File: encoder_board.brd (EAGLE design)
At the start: 39 x 43.2 mm, 13 parts, among them J1 1X2-3.5MM, J2 1X2-3.5MM, J3 1X2-3.5MM, Q1 BSS138, Q2 BSS138, Q3 BSS138, U1 ATTINY85-20P

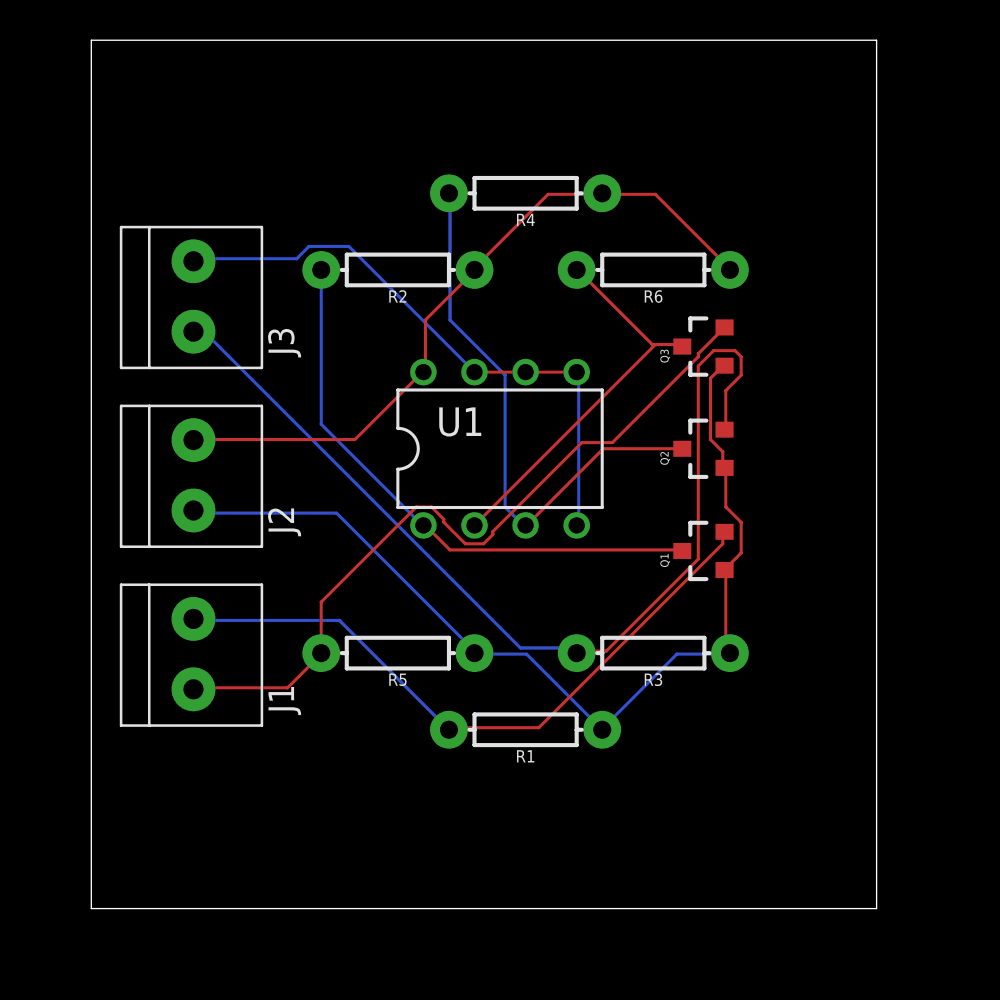
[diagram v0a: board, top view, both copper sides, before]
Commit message: Add files via upload
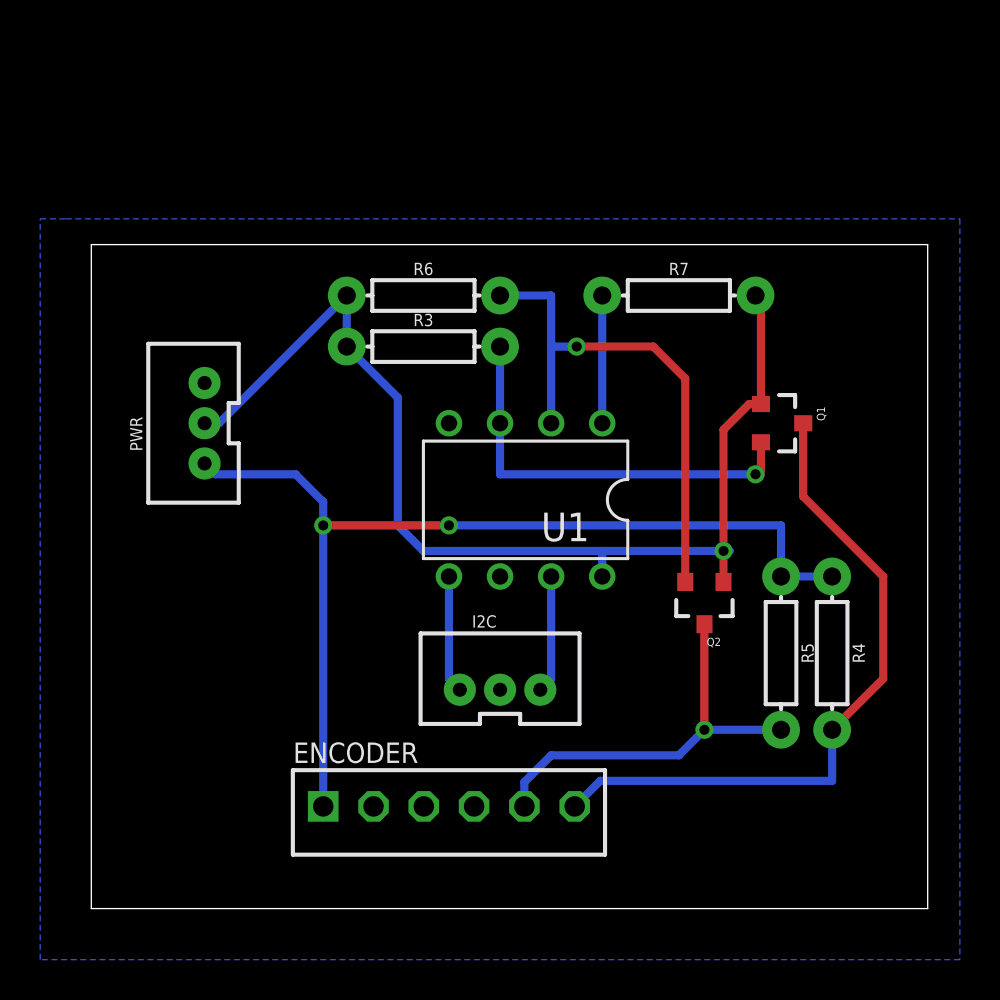
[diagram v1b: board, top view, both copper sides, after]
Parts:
- removed J1, J2, J3: 1X2-3.5MM, adafruit:1X2-3.5MM
- removed Q3: BSS138, SparkFun:SOT23-3
- removed R1, R2: 10k, SparkFun-Resistors:AXIAL-0.3
- added ENCODER: (no value), con-jst-eh:B6B-EH-A
- added I2C, PWR: (no value), SparkFun-Connectors:JST-3-PTH-VERT
- added R7: 10k, SparkFun-Resistors:AXIAL-0.3
- moved R4 27.5 mm to (36.8, 12.7), turned to 270 degrees
- moved R3 19.1 mm to (16.5, 27.9), turned to 0 degrees
- moved R5 19.0 mm to (34.3, 12.7), turned to 270 degrees
- moved R6 11.5 mm to (16.5, 30.5), turned to 0 degrees
- moved Q2 7.62 mm to (30.5, 15.2), turned to 180 degrees
- moved Q1 7.41 mm to (34.3, 24.1), turned to 270 degrees
- moved U1 2.84 mm to (21.6, 20.3), turned to 180 degrees
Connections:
- removed net 5V: J2.2, R2.P$1, R4.P$1, R6.P$1, U1.8
- removed net CLK3.3V: J1.1, Q3.2, R5.P$2
- removed net CLK5V: Q3.3, R6.P$2, U1.2
- removed net DATA3.3V: J3.1, Q2.2, R3.P$2
- removed net DATA5V: Q2.3, R4.P$2, U1.3
- removed net INT3.3V: J1.2, Q1.2, R1.P$2
- removed net INT5V: Q1.3, R2.P$2, U1.1
- new net 12V: ENCODER.1, PWR.1, R4.P$1, R5.P$1
- new net CHAN_A3.3V: Q1.2, R3.P$2, U1.3
- new net CHAN_A5V: ENCODER.6, Q1.3, R4.P$2
- new net CHAN_B3.3V: Q2.2, R6.P$2, U1.2
- new net CHAN_B5V: ENCODER.5, Q2.3, R5.P$2
- new net N$1: R7.P$1, U1.1
- new net SCK: I2C.3, U1.7
- new net SDA: I2C.1, U1.5
- net 3.3V: now also PWR.2, R6.P$1, R7.P$2, U1.8; no longer J2.1, Q3.1, R1.P$1, R5.P$1
- net GND: now also ENCODER.2, ENCODER.3, ENCODER.4, I2C.2, PWR.3; no longer J3.2, U1.5, U1.7
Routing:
- net DATA3.3V: track 49.8 -> 0.00 mm
- net 12V: track 0.00 -> 49.7 mm, vias 0 -> 2
- net CLK3.3V: track 37.1 -> 0.00 mm
- net 5V: track 34.9 -> 0.00 mm
- net CHAN_A5V: track 0.00 -> 33.8 mm
- net INT3.3V: track 33.1 -> 0.00 mm
- net GND: track 29.8 -> 0.00 mm
- net INT5V: track 28.2 -> 0.00 mm
- net DATA5V: track 27.5 -> 0.00 mm
- net CHAN_B3.3V: track 0.00 -> 26.3 mm, vias 0 -> 1
- net CHAN_A3.3V: track 0.00 -> 20.9 mm, vias 0 -> 1
- net CHAN_B5V: track 0.00 -> 20.3 mm, vias 0 -> 1
- net CLK5V: track 19.5 -> 0.00 mm
- net 3.3V: track 48.6 -> 56.0 mm, vias 0 -> 1
- net N$1: track 0.00 -> 6.35 mm
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- added copper zone on layer 16, net GND
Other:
- board size 39 x 43.2 mm -> 41.6 x 33 mm
